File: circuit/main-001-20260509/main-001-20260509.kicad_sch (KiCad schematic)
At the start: 20 parts, among them J1 Conn_Relay, J2 Conn_Sub, Q1 BSS138, Q2 BSS138, SW1 RESET, U1 DEV-16771, U2 BNO055

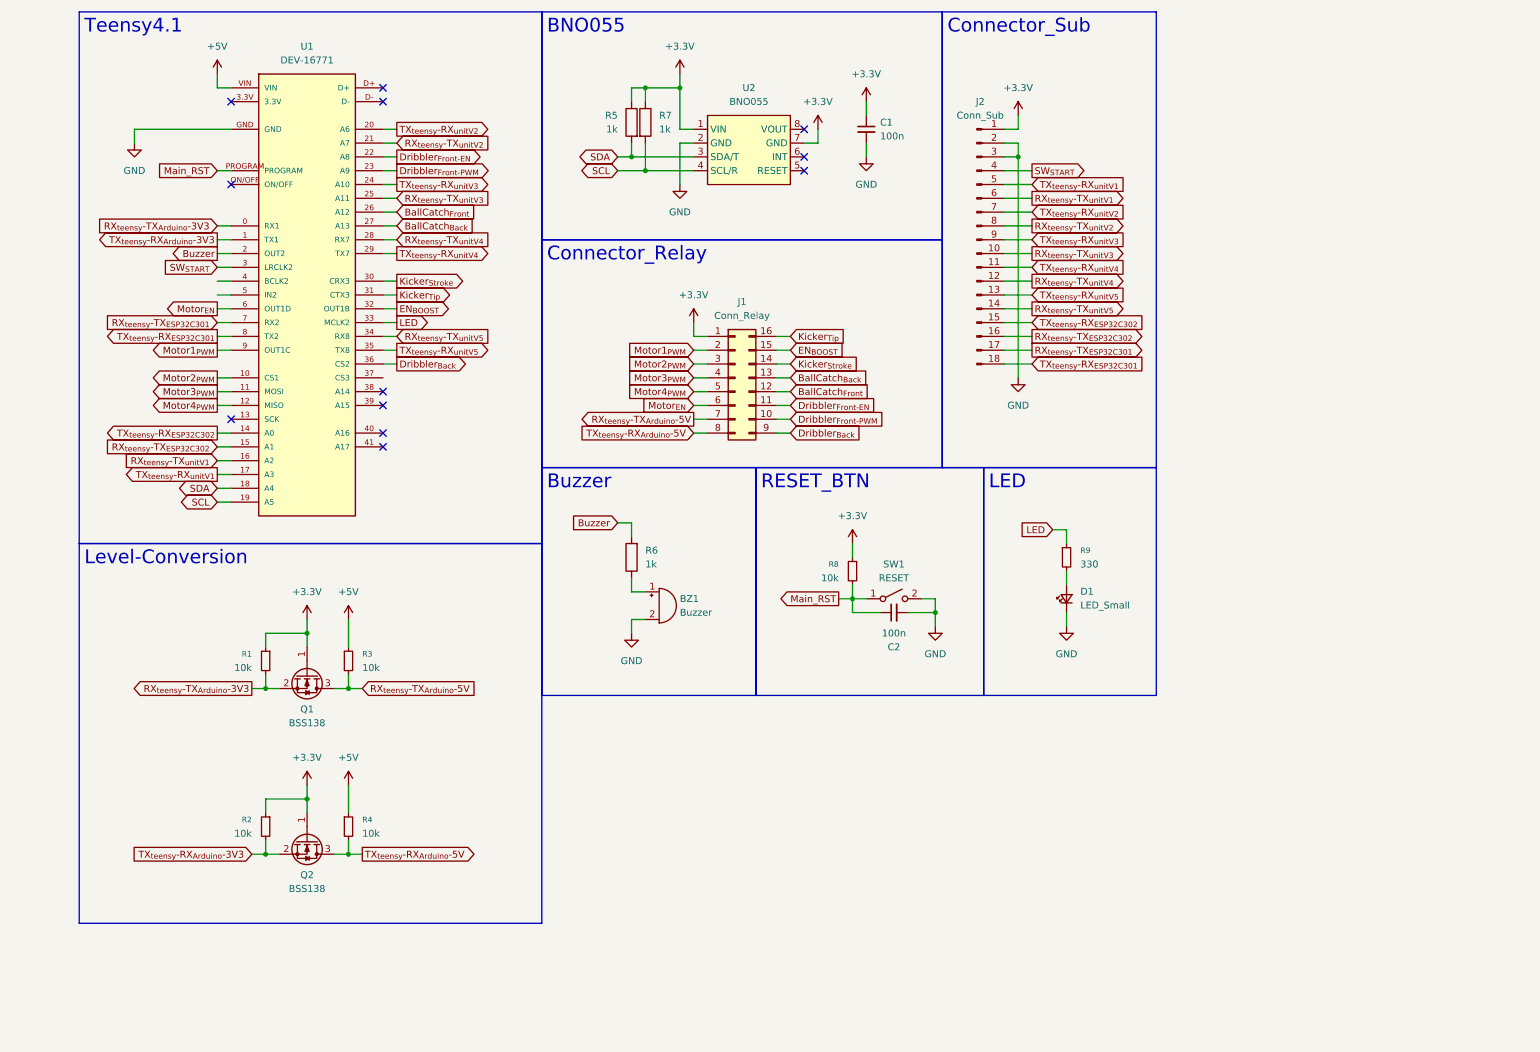
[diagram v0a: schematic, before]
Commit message: Update メイン基板のPCB完成
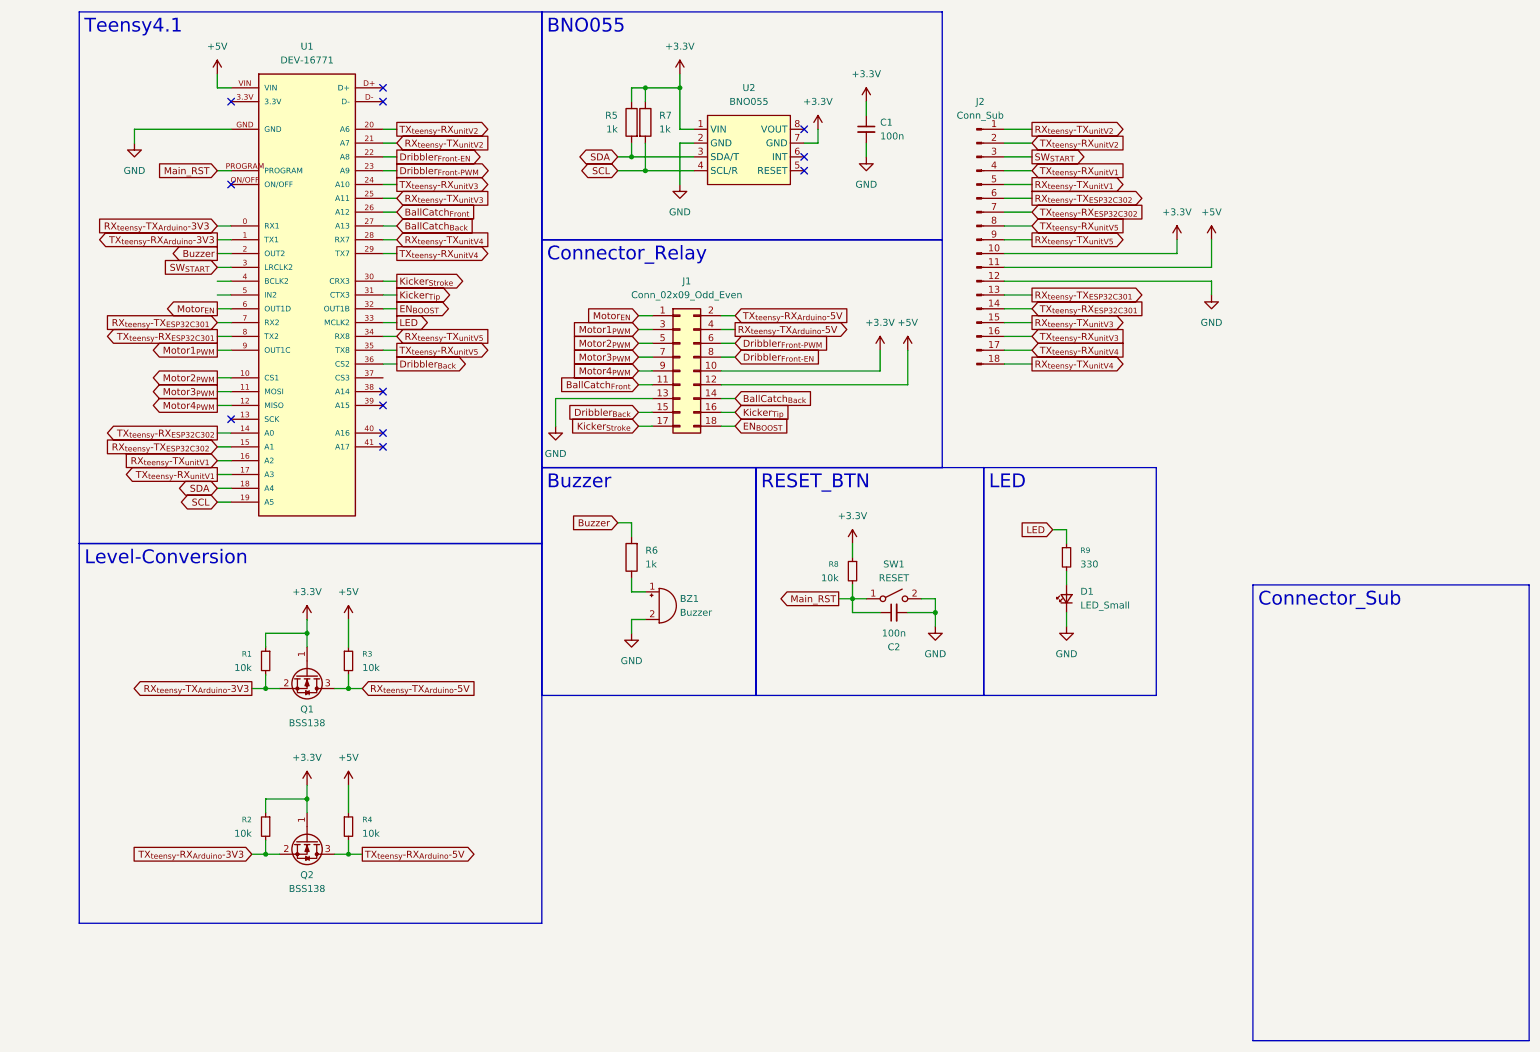
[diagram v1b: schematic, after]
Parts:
- removed J1: Conn_Relay, Connector_PinSocket_2.54mm:PinSocket_2x08_P2.54mm_Vertical, symbol Connector_Generic:Conn_02x08_Counter_Clockwise
- added J1: Conn_02x09_Odd_Even, Connector_PinHeader_2.54mm:PinHeader_2x09_P2.54mm_Vertical, symbol Connector_Generic:Conn_02x09_Odd_Even
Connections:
- net +3.3V: now also J2.10 (Pin_10), J1.10 (Pin_10); no longer J2.1 (Pin_1)
- net +5V: now also J2.11 (Pin_11), J1.12 (Pin_12)
- net BallCatch_{Back}: now also J1.14 (Pin_14)
- net BallCatch_{Front}: now also J1.11 (Pin_11)
- net Dribbler_{Back}: now also J1.15 (Pin_15)
- net Dribbler_{Front-EN}: now also J1.8 (Pin_8)
- net Dribbler_{Front-PWM}: now also J1.6 (Pin_6)
- net EN_{BOOST}: now also J1.18 (Pin_18)
- net GND: now also J2.12 (Pin_12), J1.13 (Pin_13); no longer J2.2 (Pin_2), J2.3 (Pin_3)
- net Kicker_{Stroke}: now also J1.17 (Pin_17)
- net Kicker_{Tip}: now also J1.16 (Pin_16)
- net Motor1_{PWM}: now also J1.3 (Pin_3)
- net Motor2_{PWM}: now also J1.5 (Pin_5)
- net Motor3_{PWM}: now also J1.7 (Pin_7)
- net Motor4_{PWM}: now also J1.9 (Pin_9)
- net Motor_{EN}: now also J1.1 (Pin_1)
- net RX_{teensy}-TX_{Arduino}-5V: now also J1.4 (Pin_4)
- net RX_{teensy}-TX_{ESP32C301}: now also J2.13 (Pin_13); no longer J2.17 (Pin_17)
- net RX_{teensy}-TX_{ESP32C302}: now also J2.6 (Pin_6); no longer J2.16 (Pin_16)
- net RX_{teensy}-TX_{unitV1}: now also J2.5 (Pin_5); no longer J2.6 (Pin_6)
- net RX_{teensy}-TX_{unitV2}: now also J2.1 (Pin_1); no longer J2.8 (Pin_8)
- net RX_{teensy}-TX_{unitV3}: now also J2.15 (Pin_15); no longer J2.10 (Pin_10)
- net RX_{teensy}-TX_{unitV4}: now also J2.18 (Pin_18); no longer J2.12 (Pin_12)
- net RX_{teensy}-TX_{unitV5}: now also J2.9 (Pin_9); no longer J2.14 (Pin_14)
- net SW_{START}: now also J2.3 (Pin_3); no longer J2.4 (Pin_4)
- net TX_{teensy}-RX_{Arduino}-5V: now also J1.2 (Pin_2)
- net TX_{teensy}-RX_{ESP32C301}: now also J2.14 (Pin_14); no longer J2.18 (Pin_18)
- net TX_{teensy}-RX_{ESP32C302}: now also J2.7 (Pin_7); no longer J2.15 (Pin_15)
- net TX_{teensy}-RX_{unitV1}: now also J2.4 (Pin_4); no longer J2.5 (Pin_5)
- net TX_{teensy}-RX_{unitV2}: now also J2.2 (Pin_2); no longer J2.7 (Pin_7)
- net TX_{teensy}-RX_{unitV3}: now also J2.16 (Pin_16); no longer J2.9 (Pin_9)
- net TX_{teensy}-RX_{unitV4}: now also J2.17 (Pin_17); no longer J2.11 (Pin_11)
- net TX_{teensy}-RX_{unitV5}: now also J2.8 (Pin_8); no longer J2.13 (Pin_13)

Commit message: Update メイン基板をDRした
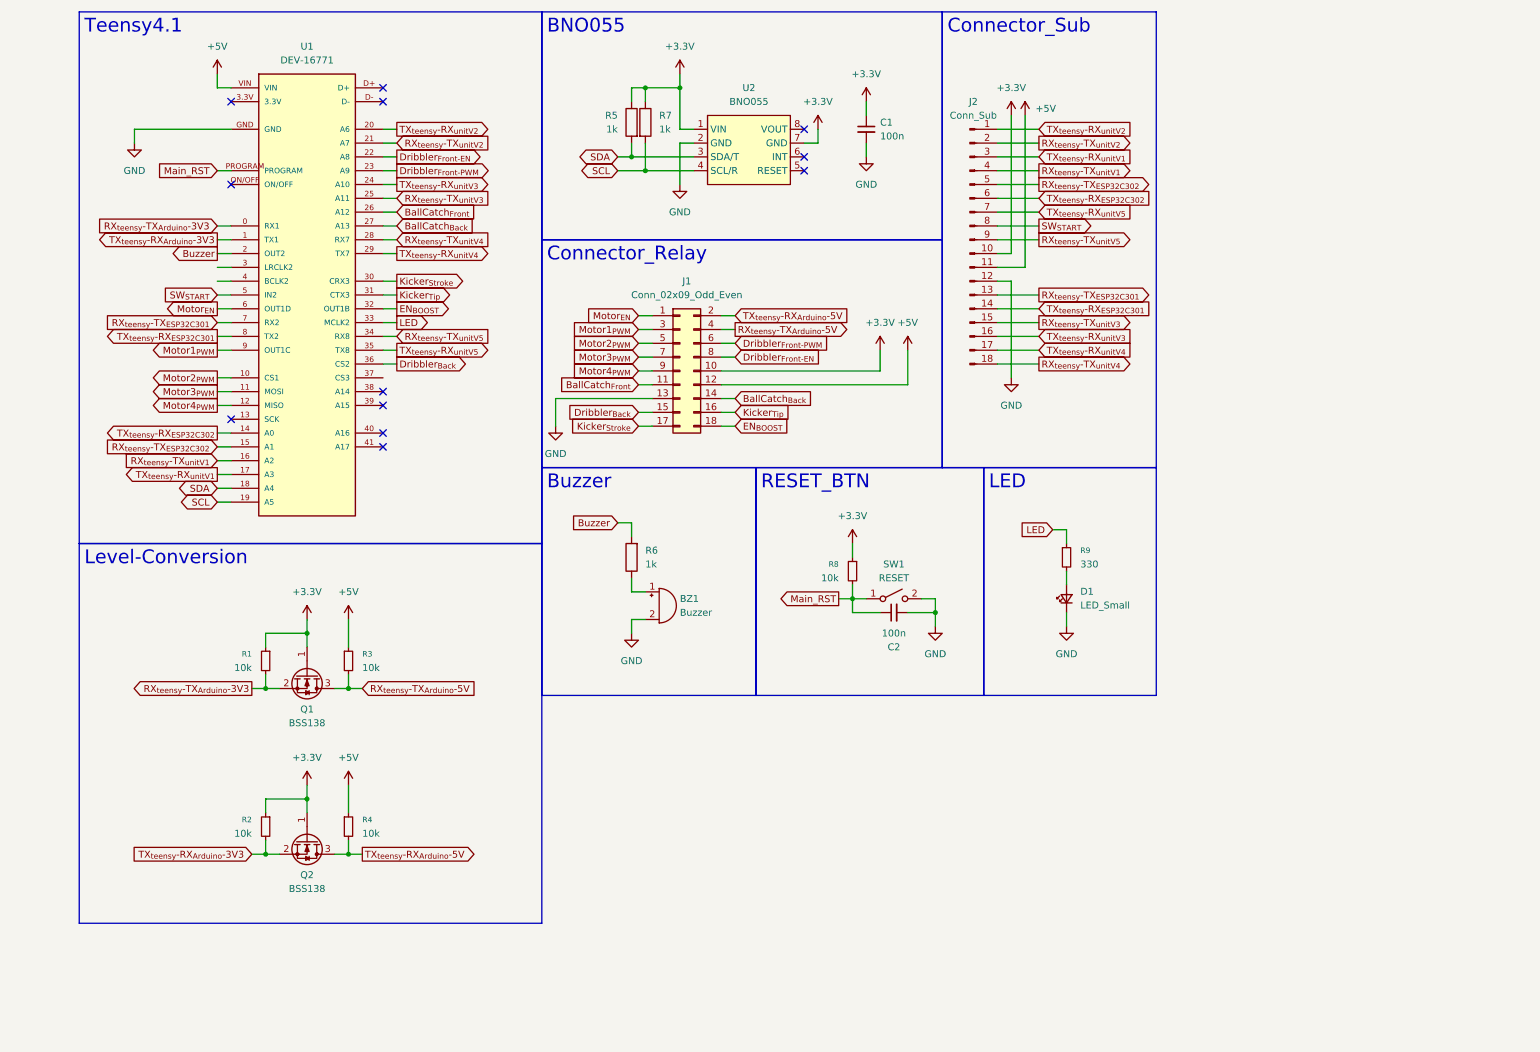
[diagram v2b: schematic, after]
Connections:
- net RX_{teensy}-TX_{ESP32C302}: now also J2.5 (Pin_5); no longer J2.6 (Pin_6)
- net RX_{teensy}-TX_{unitV1}: now also J2.4 (Pin_4); no longer J2.5 (Pin_5)
- net RX_{teensy}-TX_{unitV2}: now also J2.2 (Pin_2); no longer J2.1 (Pin_1)
- net SW_{START}: now also J2.8 (Pin_8), U1.5 (IN2); no longer J2.3 (Pin_3), U1.3 (LRCLK2)
- net TX_{teensy}-RX_{ESP32C302}: now also J2.6 (Pin_6); no longer J2.7 (Pin_7)
- net TX_{teensy}-RX_{unitV1}: now also J2.3 (Pin_3); no longer J2.4 (Pin_4)
- net TX_{teensy}-RX_{unitV2}: now also J2.1 (Pin_1); no longer J2.2 (Pin_2)
- net TX_{teensy}-RX_{unitV5}: now also J2.7 (Pin_7); no longer J2.8 (Pin_8)
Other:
- moved on the sheet: J2
